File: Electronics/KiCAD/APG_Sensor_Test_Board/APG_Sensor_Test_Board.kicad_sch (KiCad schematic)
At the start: 0 parts

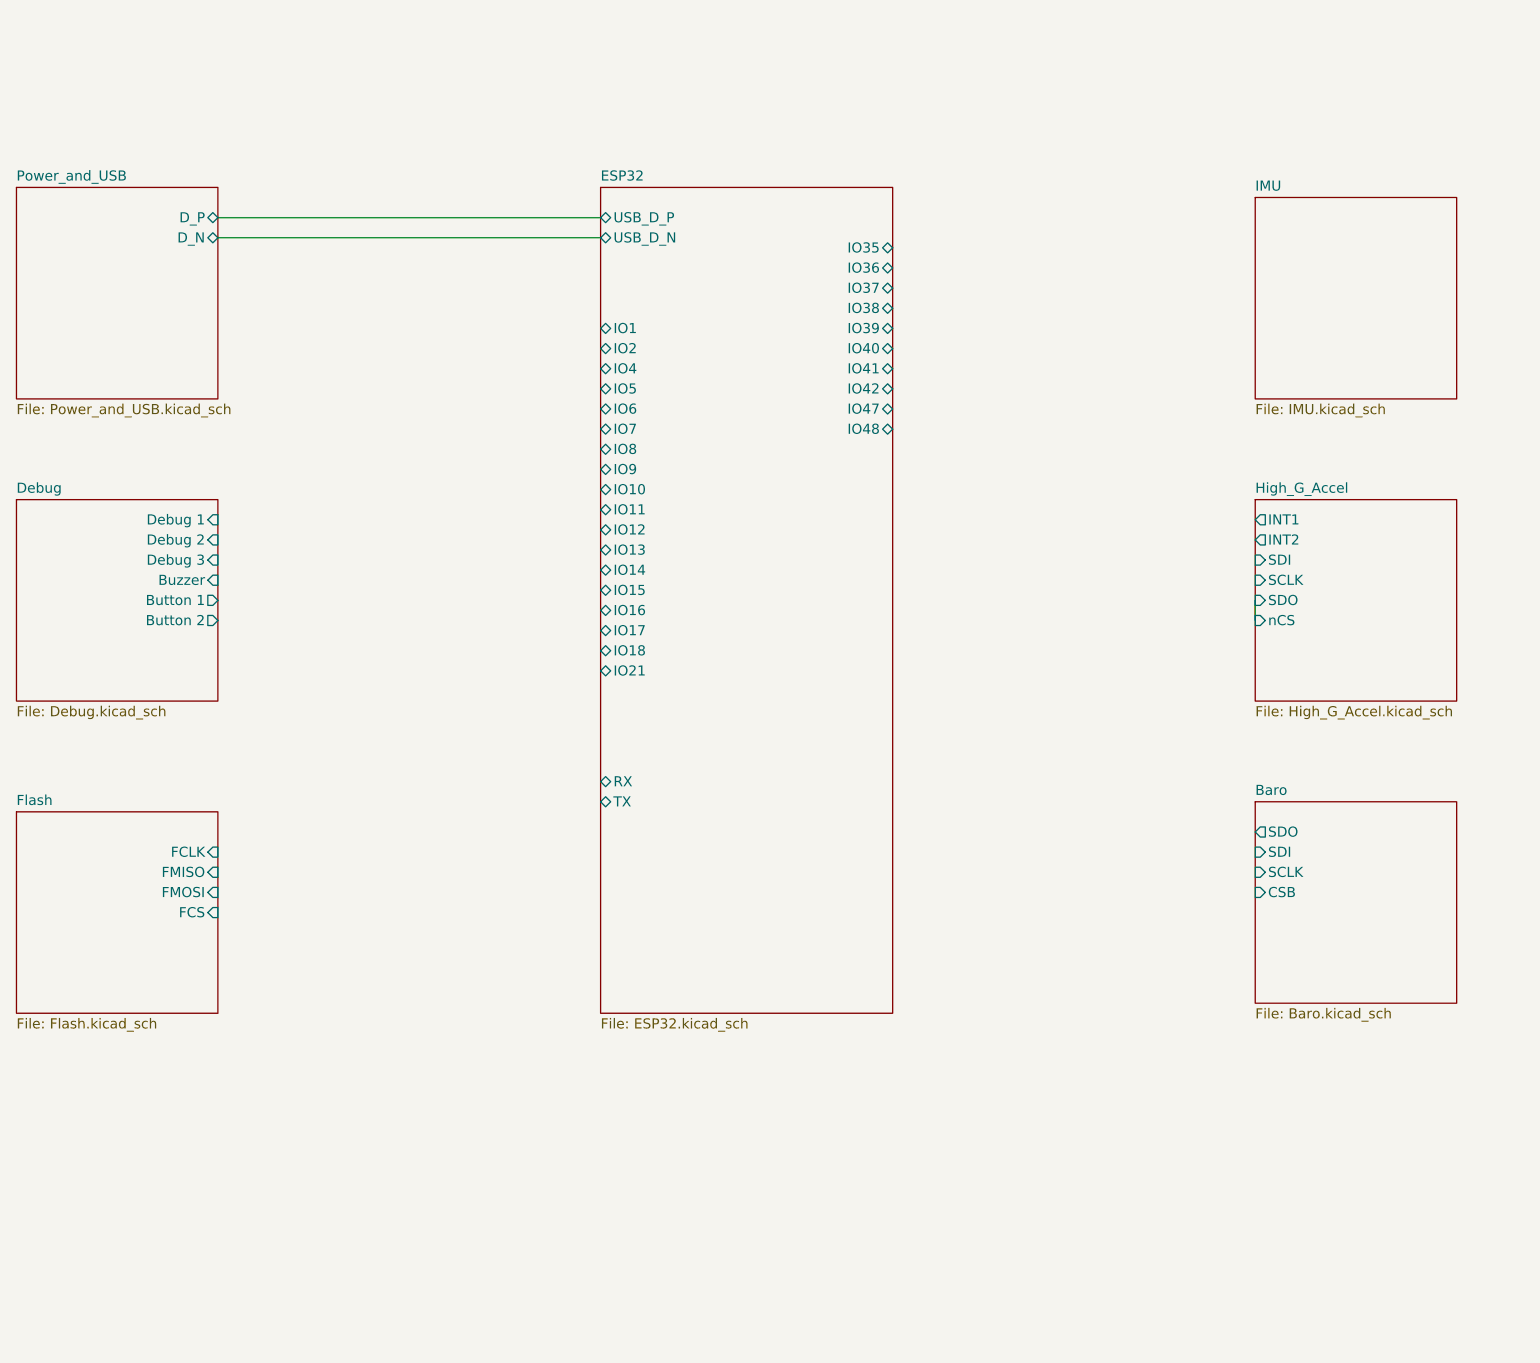
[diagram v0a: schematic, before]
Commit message: Main Schematic Complete
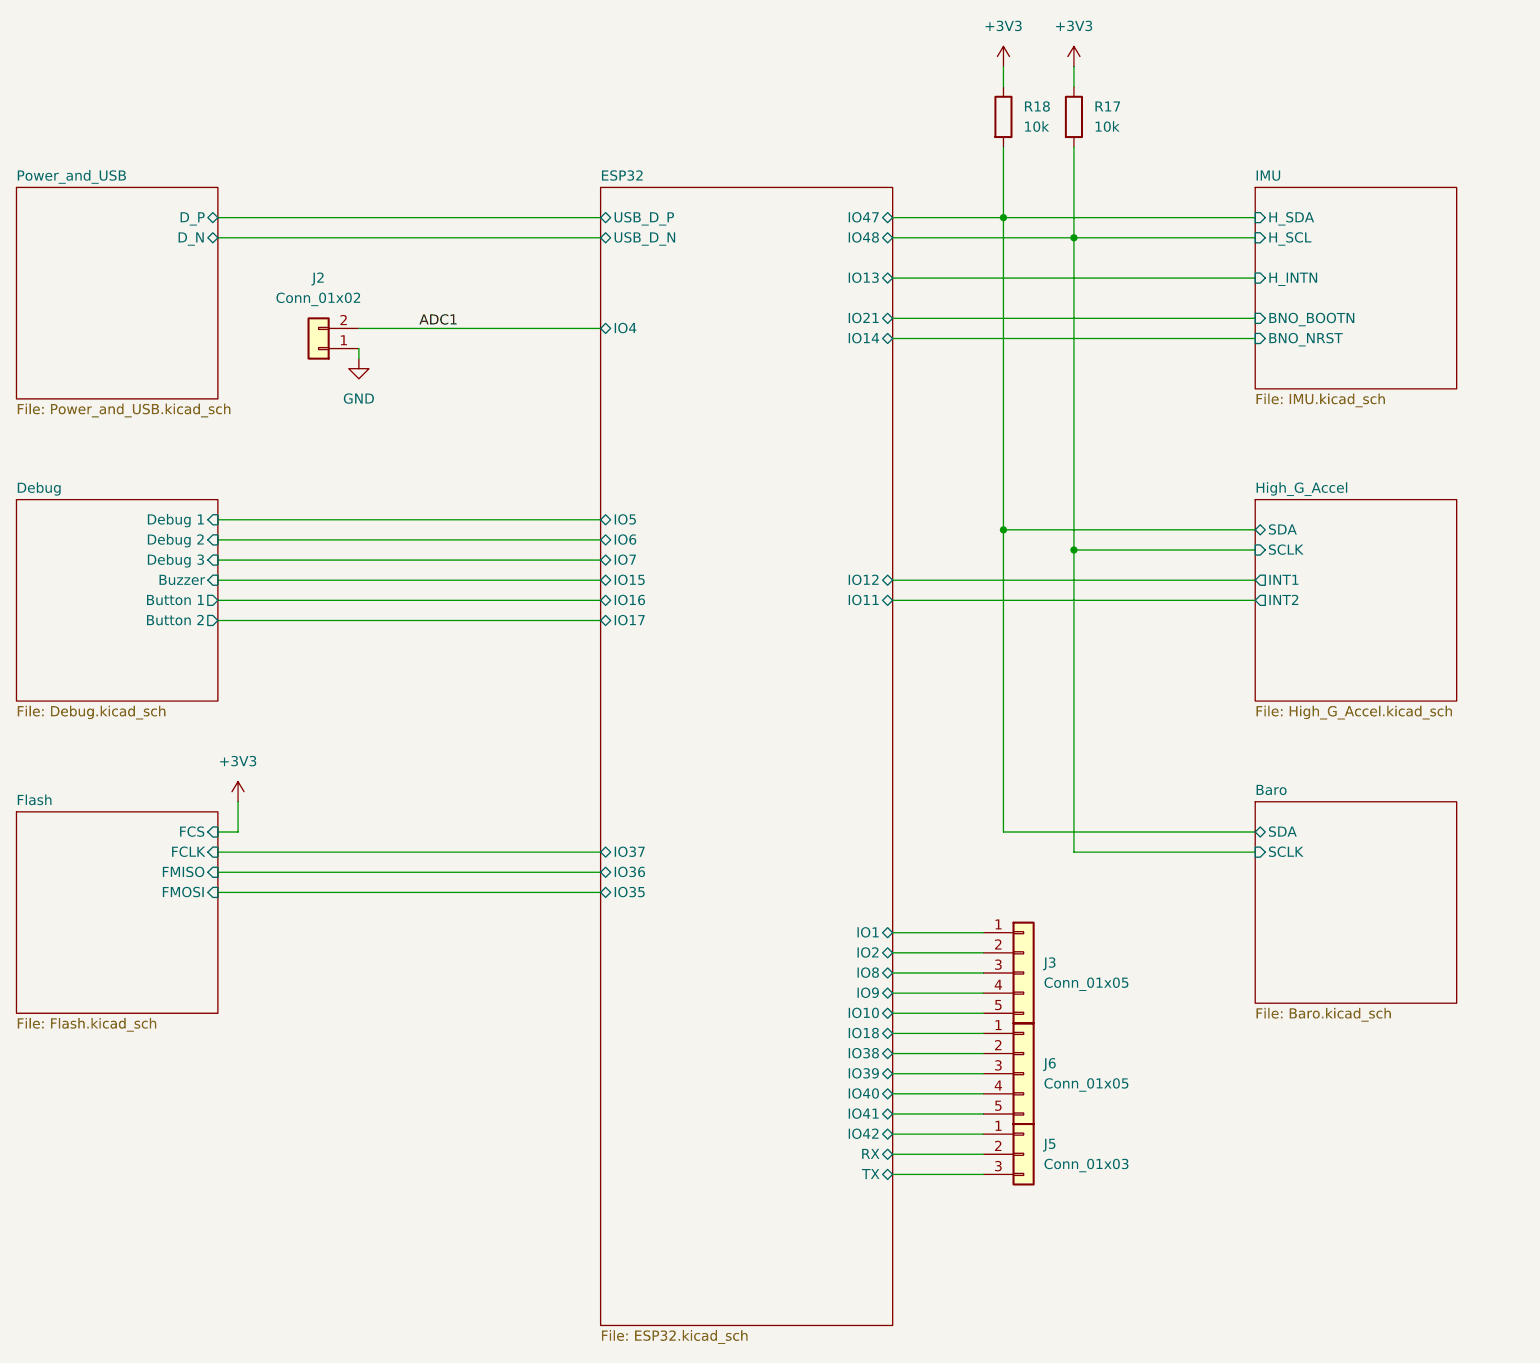
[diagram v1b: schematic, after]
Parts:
- added J2: Conn_01x02, symbol Connector_Generic:Conn_01x02
- added J3, J6: Conn_01x05, symbol Connector_Generic:Conn_01x05
- added J5: Conn_01x03, symbol Connector_Generic:Conn_01x03
- added R17, R18: 10k, symbol Device:R
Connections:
- net Baro/SCLK: now also R17.2
- net ESP32/IO1: now also J3.1 (Pin_1)
- net ESP32/IO10: now also J3.5 (Pin_5)
- net ESP32/IO18: now also J6.1 (Pin_1)
- net ESP32/IO2: now also J3.2 (Pin_2)
- net ESP32/IO38: now also J6.2 (Pin_2)
- net ESP32/IO39: now also J6.3 (Pin_3)
- net ESP32/IO40: now also J6.4 (Pin_4)
- net ESP32/IO41: now also J6.5 (Pin_5)
- net ESP32/IO42: now also J5.1 (Pin_1)
- net ESP32/IO8: now also J3.3 (Pin_3)
- net ESP32/IO9: now also J3.4 (Pin_4)
- net ESP32/RX: now also J5.2 (Pin_2)
- net ESP32/TX: now also J5.3 (Pin_3)
- new net +3V3: R17.1, R18.1
- new net ADC1: J2.2 (Pin_2)
- new net Baro/SDA: R18.2
- new net GND: J2.1 (Pin_1)
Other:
- sheet Baro ports: added SDA; removed CSB, SDI, SDO
- sheet High_G_Accel ports: added SDA; removed SDI, SDO, nCS
- sheet IMU ports: added BNO_BOOTN, BNO_NRST, H_INTN, H_SCL, H_SDA; removed none
